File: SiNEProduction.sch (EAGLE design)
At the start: 39 parts, among them IC1 74HCT164D, IC3 ATTINY24/44/84-SSU, J1 AVR_SPI_PRG_6NS

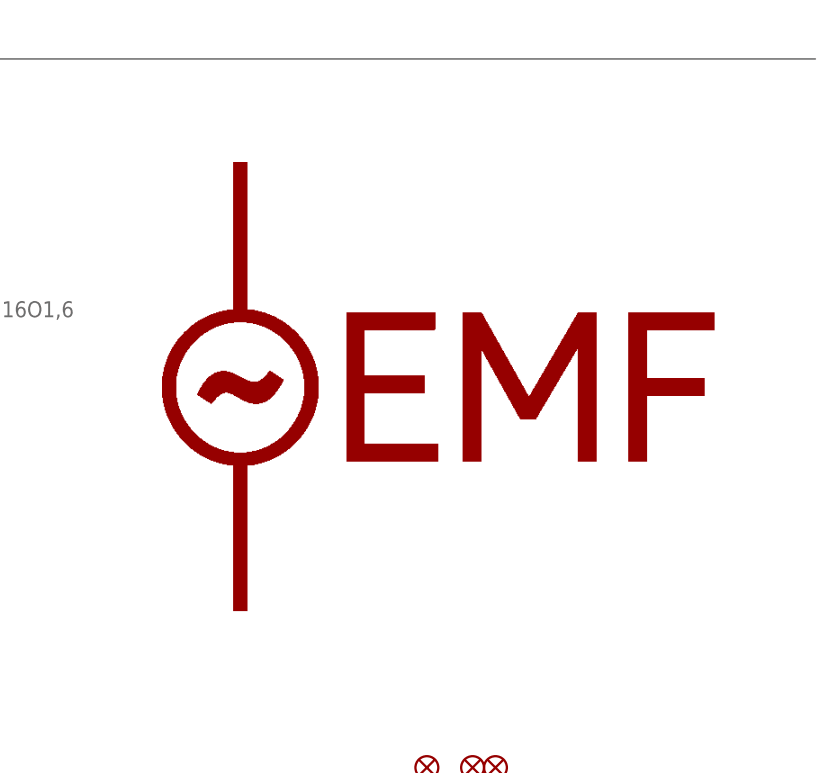
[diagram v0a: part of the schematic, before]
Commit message: Last tweaks for EMF Logo
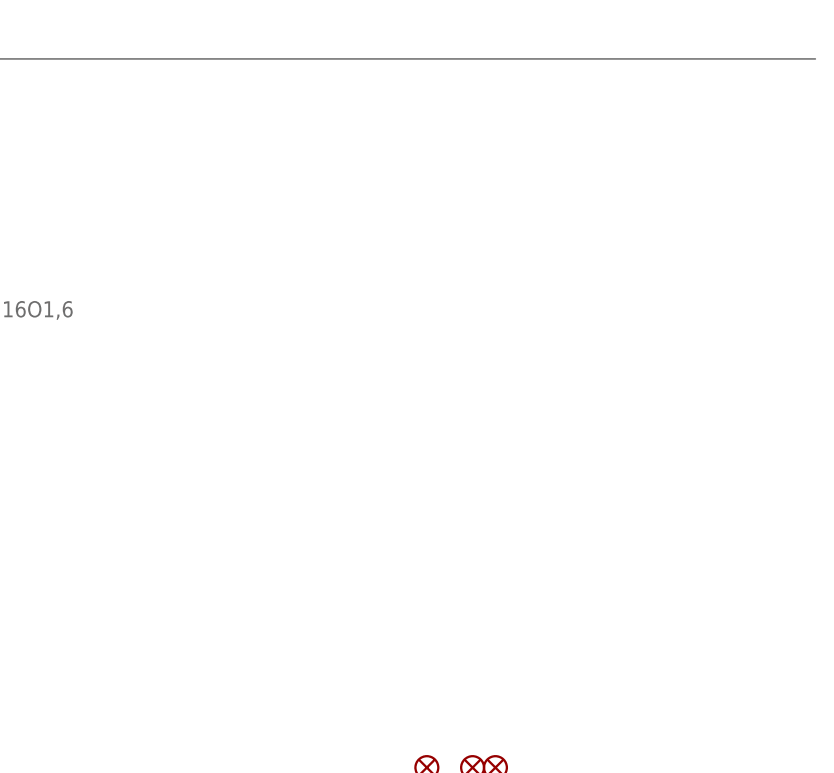
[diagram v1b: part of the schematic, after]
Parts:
- removed U$2: MINIEMF, TiLDA:MINIEMF
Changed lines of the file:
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@@
 <grid distance="0.1" unitdist="inch" unit="inch" style="lines" multiple="1" display="no" altdistance="0.01" altunitdist="inch" altunit="inch"/>
 <layers>
-<layer number="1" name="Top" color="4" fill="1" visible="yes" active="no"/>
-<layer number="2" name="Route2" color="1" fill="3" visible="yes" active="no"/>
-<layer number="3" name="Route3" color="4" fill="3" visible="yes" active="no"/>
-<layer number="4" name="Route4" color="1" fill="4" visible="yes" active="no"/>
-<layer number="5" name="Route5" color="4" fill="4" visible="yes" active="no"/>
-<layer number="6" name="Route6" color="1" fill="8" visible="yes" active="no"/>
-<layer number="7" name="Route7" color="4" fill="8" visible="yes" active="no"/>
-<layer number="8" name="Route8" color="1" fill="2" visible="yes" active="no"/>
-<layer number="9" name="Route9" color="4" fill="2" visible="yes" active="no"/>
-<layer number="10" name="Route10" color="1" fill="7" visible="yes" active="no"/>
-<layer number="11" name="Route11" color="4" fill="7" visible="yes" active="no"/>
-<layer number="12" name="Route12" color="1" fill="5" visible="yes" active="no"/>
-<layer number="13" name="Route13" color="4" fill="5" visible="yes" active="no"/>
-<layer number="14" name="Route14" color="1" fill="6" visible="yes" active="no"/>
-<layer number="15" name="Route15" color="4" fill="6" visible="yes" active="no"/>
-<layer number="16" name="Bottom" color="1" fill="1" visible="yes" active="no"/>
-<layer number="17" name="Pads" color="2" fill="1" visible="yes" active="no"/>
-<layer number="18" name="Vias" color="2" fill="1" visible="yes" active="no"/>
-<layer number="19" name="Unrouted" color="6" fill="1" visible="yes" active="no"/>
-<layer number="20" name="Dimension" color="15" fill="1" visible="yes" active="no"/>
-<layer number="21" name="tPlace" color="7" fill="1" visible="yes" active="no"/>
-<layer number="22" name="bPlace" color="14" fill="1" visible="yes" active="no"/>
-<layer number="23" name="tOrigins" color="15" fill="1" visible="yes" active="no"/>
-<layer number="24" name="bOrigins" color="15" fill="1" visible="yes" active="no"/>
-<layer number="25" name="tNames" color="7" fill="1" visible="yes" active="no"/>
-<layer number="26" name="bNames" color="7" fill="1" visible="yes" active="no"/>
-<layer number="27" name="tValues" color="7" fill="1" visible="yes" active="no"/>
-<layer number="28" name="bValues" color="7" fill="1" visible="yes" active="no"/>
+<layer number="1" name="Top" color="4" fill="1" visible="no" active="no"/>
+<layer number="2" name="Route2" color="1" fill="3" visible="no" active="no"/>
+<layer number="3" name="Route3" color="4" fill="3" visible="no" active="no"/>
+<layer number="4" name="Route4" color="1" fill="4" visible="no" active="no"/>
+<layer number="5" name="Route5" color="4" fill="4" visible="no" active="no"/>
+<layer number="6" name="Route6" color="1" fill="8" visible="no" active="no"/>
+<layer number="7" name="Route7" color="4" fill="8" visible="no" active="no"/>
+<layer number="8" name="Route8" color="1" fill="2" visible="no" active="no"/>
+<layer number="9" name="Route9" color="4" fill="2" visible="no" active="no"/>
+<layer number="10" name="Route10" color="1" fill="7" visible="no" active="no"/>
+<layer number="11" name="Route11" color="4" fill="7" visible="no" active="no"/>
+<layer number="12" name="Route12" color="1" fill="5" visible="no" active="no"/>
+<layer number="13" name="Route13" color="4" fill="5" visible="no" active="no"/>
+<layer number="14" name="Route14" color="1" fill="6" visible="no" active="no"/>
+<layer number="15" name="Route15" color="4" fill="6" visible="no" active="no"/>
+<layer number="16" name="Bottom" color="1" fill="1" visible="no" active="no"/>
+<layer number="17" name="Pads" color="2" fill="1" visible="no" active="no"/>
+<layer number="18" name="Vias" color="2" fill="1" visible="no" active="no"/>
+<layer number="19" name="Unrouted" color="6" fill="1" visible="no" active="no"/>
+<layer number="20" name="Dimension" color="15" fill="1" visible="no" active="no"/>
+<layer number="21" name="tPlace" color="7" fill="1" visible="no" active="no"/>
+<layer number="22" name="bPlace" color="14" fill="1" visible="no" active="no"/>
+<layer number="23" name="tOrigins" color="15" fill="1" visible="no" active="no"/>
+<layer number="24" name="bOrigins" color="15" fill="1" visible="no" active="no"/>
+<layer number="25" name="tNames" color="7" fill="1" visible="no" active="no"/>
+<layer number="26" name="bNames" color="7" fill="1" visible="no" active="no"/>
+<layer number="27" name="tValues" color="7" fill="1" visible="no" active="no"/>
+<layer number="28" name="bValues" color="7" fill="1" visible="no" active="no"/>
 <layer number="29" name="tStop" color="7" fill="3" visible="no" active="no"/>
 <layer number="30" name="bStop" color="7" fill="6" visible="no" active="no"/>
@@
 <layer number="35" name="tGlue" color="7" fill="4" visible="no" active="no"/>
 <layer number="36" name="bGlue" color="7" fill="5" visible="no" active="no"/>
-<layer number="37" name="tTest" color="7" fill="1" visible="yes" active="no"/>
-<layer number="38" name="bTest" color="7" fill="1" visible="yes" active="no"/>
+<layer number="37" name="tTest" color="7" fill="1" visible="no" active="no"/>
+<layer number="38" name="bTest" color="7" fill="1" visible="no" active="no"/>
 <layer number="39" name="tKeepout" color="4" fill="11" visible="no" active="no"/>
 <layer number="40" name="bKeepout" color="1" fill="11" visible="no" active="no"/>
@@
 <layer number="44" name="Drills" color="7" fill="1" visible="no" active="no"/>
 <layer number="45" name="Holes" color="7" fill="1" visible="no" active="no"/>
-<layer number="46" name="Milling" color="3" fill="1" visible="yes" active="no"/>
-<layer number="47" name="Measures" color="7" fill="1" visible="yes" active="no"/>
-<layer number="48" name="Document" color="7" fill="1" visible="yes" active="no"/>
-<layer number="49" name="Reference" color="13" fill="1" visible="yes" active="no"/>
-<layer number="50" name="dxf" color="7" fill="1" visible="yes" active="no"/>
-<layer number="51" name="tDocu" color="14" fill="1" visible="yes" active="no"/>
-<layer number="52" name="bDocu" color="7" fill="1" visible="yes" active="no"/>
-<layer number="53" name="tGND_GNDA" color="7" fill="9" visible="yes" active="no"/>
-<layer number="54" name="bGND_GNDA" color="1" fill="9" visible="yes" active="no"/>
-<layer number="56" name="wert" color="7" fill="1" visible="yes" active="no"/>
+<layer number="46" name="Milling" color="3" fill="1" visible="no" active="no"/>
+<layer number="47" name="Measures" color="7" fill="1" visible="no" active="no"/>
+<layer number="48" name="Document" color="7" fill="1" visible="no" active="no"/>
+<layer number="49" name="Reference" color="13" fill="1" visible="no" active="no"/>
+<layer number="50" name="dxf" color="7" fill="1" visible="no" active="no"/>
+<layer number="51" name="tDocu" color="14" fill="1" visible="no" active="no"/>
+<layer number="52" name="bDocu" color="7" fill="1" visible="no" active="no"/>
+<layer number="53" name="tGND_GNDA" color="7" fill="9" visible="no" active="no"/>
+<layer number="54" name="bGND_GNDA" color="1" fill="9" visible="no" active="no"/>
+<layer number="56" name="wert" color="7" fill="1" visible="no" active="no"/>
 <layer number="91" name="Nets" color="2" fill="1" visible="yes" active="yes"/>
 <layer number="92" name="Busses" color="1" fill="1" visible="yes" active="yes"/>
@@
 <part name="TP2" library="SiNE Parts" deviceset="TP" device="B2,54"/>
 <part name="IC1" library="SiNE Parts" deviceset="74*164" device="D" technology="HCT"/>
-<part name="U$2" library="TiLDA" deviceset="MINIEMF" device=""/>
 <part name="U$3" library="SiNE Parts" deviceset="IR-RECEIVE-COMBINED" device=""/>
 <part name="PAD1" library="wirepad" deviceset="WIREPAD" device="4,16O1,6"/>
@@
 <instance part="TP2" gate="G$1" x="129.54" y="114.3"/>
 <instance part="IC1" gate="A" x="139.7" y="147.32"/>
-<instance part="U$2" gate="G$1" x="190.5" y="40.64"/>
 <instance part="U$3" gate="G$1" x="43.18" y="78.74" rot="MR0"/>
 <instance part="PAD1" gate="G$1" x="162.56" y="78.74"/>
